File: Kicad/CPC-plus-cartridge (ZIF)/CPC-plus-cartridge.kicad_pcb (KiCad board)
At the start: 2 copper layers, 47.2 x 78.7 mm, 18 parts, among them J1 Amstrad-CPC-plus-cartridge, J2 JTAG, U1 SST39SF040, U2 XC9536XL-VQ44, U3 SPX3819M5-L-3-3, U4 XC6206PxxxMR

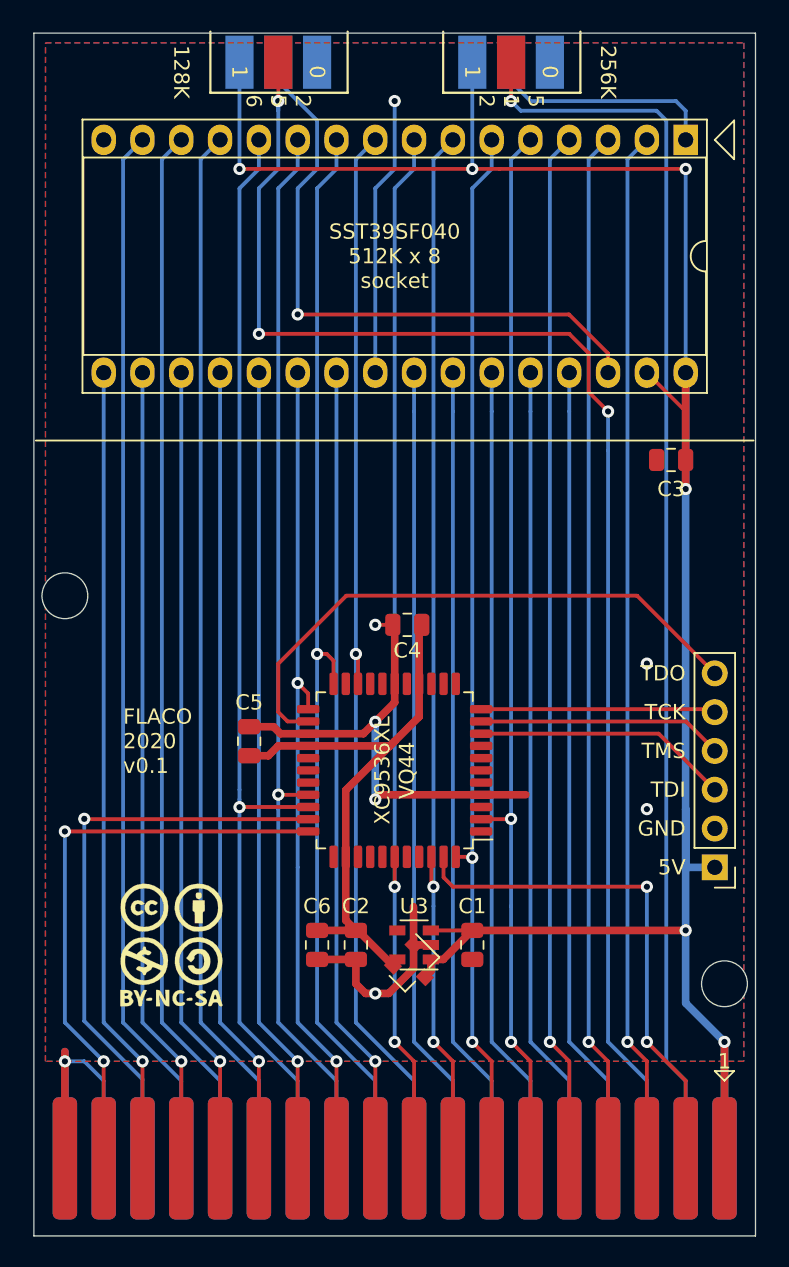
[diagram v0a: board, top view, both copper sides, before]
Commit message: Photo, InteractiveHtmlBom and README
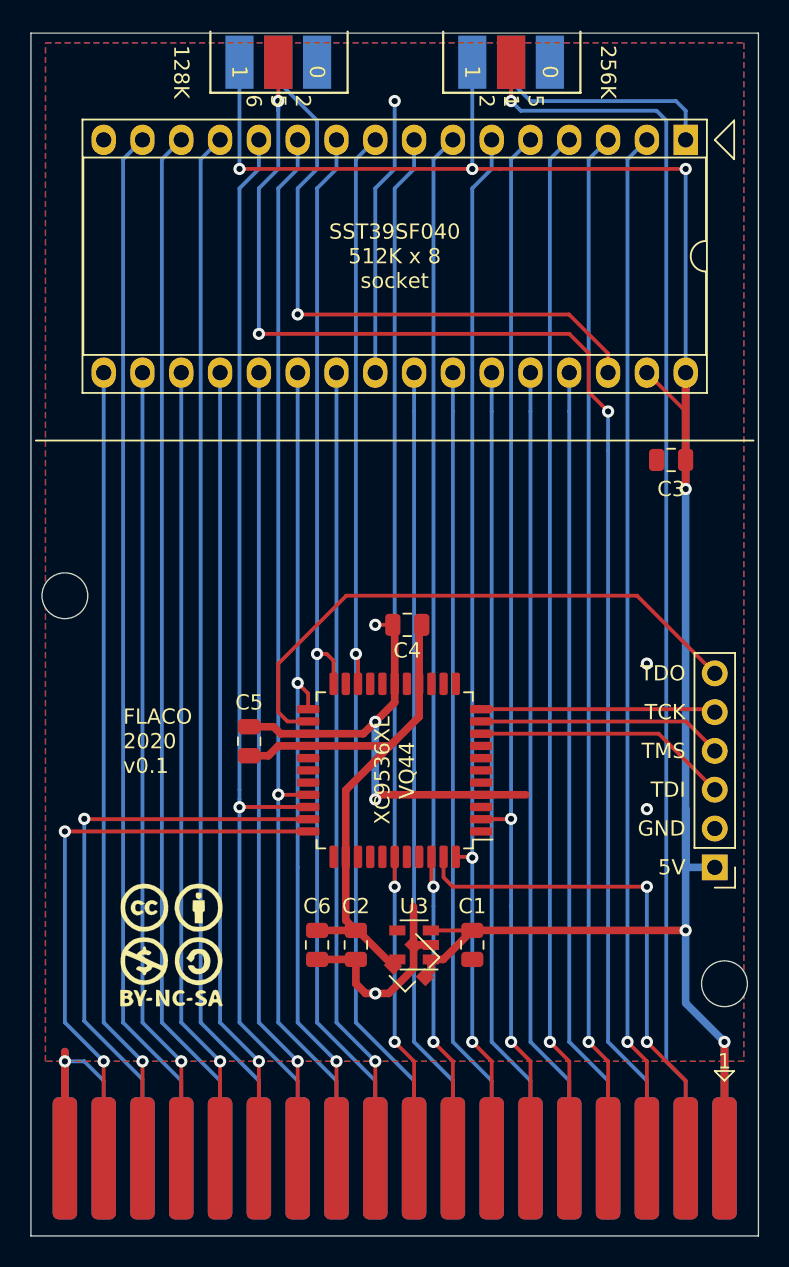
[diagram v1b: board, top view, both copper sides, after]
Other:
- board size 47.2 x 78.7 mm -> 47.6 x 78.7 mm
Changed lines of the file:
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@@
-(kicad_pcb (version 20171130) (host pcbnew 5.1.8-db9833491~88~ubuntu20.04.1)
+(kicad_pcb (version 20171130) (host pcbnew 5.1.12-84ad8e8a86~92~ubuntu20.04.1)
   (general
     (thickness 1.6)
@@
   )
   (page A4)
+  (title_block
+    (title "CPC plus cartridge (ZIF)")
+    (date 2021-12-11)
+    (rev 0.2)
+    (company "FLACO 2019-2020, licence of this schematic is CC-BY-NC-SA")
+    (comment 1 "from 0.1: slight width increase to better fit the CPC connector")
+  )
   (layers
     (0 F.Cu signal)
@@
       (effects (font (size 1 1) (thickness 0.15)))
     )
+    (fp_circle (center 0 0) (end 3 0) (layer Cmts.User) (width 0.15))
+    (fp_circle (center 0 0) (end 3.25 0) (layer F.CrtYd) (width 0.05))
     (fp_text user %R (at 0.3 0) (layer F.Fab)
       (effects (font (size 1 1) (thickness 0.15)))
     )
-    (fp_circle (center 0 0) (end 3 0) (layer Cmts.User) (width 0.15))
-    (fp_circle (center 0 0) (end 3.25 0) (layer F.CrtYd) (width 0.05))
     (pad 1 np_thru_hole circle (at 0 0) (size 3 3) (drill 3) (layers *.Cu *.Mask))
   )
@@
       (effects (font (size 1 1) (thickness 0.15)))
     )
+    (fp_circle (center 0 0) (end 3 0) (layer Cmts.User) (width 0.15))
+    (fp_circle (center 0 0) (end 3.25 0) (layer F.CrtYd) (width 0.05))
     (fp_text user %R (at 0.3 0) (layer F.Fab)
       (effects (font (size 1 1) (thickness 0.15)))
     )
-    (fp_circle (center 0 0) (end 3 0) (layer Cmts.User) (width 0.15))
-    (fp_circle (center 0 0) (end 3.25 0) (layer F.CrtYd) (width 0.05))
     (pad 1 np_thru_hole circle (at 0 0) (size 3 3) (drill 3) (layers *.Cu *.Mask))
   )
@@
       (effects (font (size 1 1) (thickness 0.15)))
     )
-    (fp_text user "PCB Edge" (at -7.54 1) (layer Dwgs.User)
-      (effects (font (size 0.5 0.5) (thickness 0.125)))
-    )
     (fp_line (start -8.54 2) (end 8.255 2) (layer Dwgs.User) (width 0.15))
     (fp_line (start -4.54 2) (end -4.54 -2) (layer F.SilkS) (width 0.15))
     (fp_line (start -4.54 -2) (end 4.445 -2) (layer F.SilkS) (width 0.15))
     (fp_line (start 4.445 -2) (end 4.445 2) (layer F.SilkS) (width 0.15))
+    (fp_text user "PCB Edge" (at -7.54 1) (layer Dwgs.User)
+      (effects (font (size 0.5 0.5) (thickness 0.125)))
+    )
     (pad 4 smd rect (at 0 0 180) (size 1.846667 3.48) (layers F.Cu F.Paste F.Mask)
       (net 31 /A18))
@@
       (effects (font (size 1 1) (thickness 0.15)))
     )
-    (fp_text user "PCB Edge" (at -7.54 1) (layer Dwgs.User)
-      (effects (font (size 0.5 0.5) (thickness 0.125)))
-    )
     (fp_line (start -8.54 2) (end 8.255 2) (layer Dwgs.User) (width 0.15))
     (fp_line (start -4.54 2) (end -4.54 -2) (layer F.SilkS) (width 0.15))
     (fp_line (start -4.54 -2) (end 4.445 -2) (layer F.SilkS) (width 0.15))
     (fp_line (start 4.445 -2) (end 4.445 2) (layer F.SilkS) (width 0.15))
+    (fp_text user "PCB Edge" (at -7.54 1) (layer Dwgs.User)
+      (effects (font (size 0.5 0.5) (thickness 0.125)))
+    )
     (pad 4 smd rect (at 0 0 180) (size 1.846667 3.48) (layers F.Cu F.Paste F.Mask)
       (net 29 /A17))
@@
     (arrow2b (pts (xy 122.555 82.55) (xy 121.968579 81.423496)))
   )
-  (gr_line (start 130.048 55.88) (end 177.292 55.88) (layer Edge.Cuts) (width 0.05))
-  (gr_line (start 130.048 134.62) (end 130.048 55.88) (layer Edge.Cuts) (width 0.05))
-  (gr_line (start 177.292 134.62) (end 177.292 55.88) (layer Edge.Cuts) (width 0.05))
+  (gr_line (start 129.8575 55.88) (end 177.4825 55.88) (layer Edge.Cuts) (width 0.05))
+  (gr_line (start 129.8575 134.62) (end 129.8575 55.88) (layer Edge.Cuts) (width 0.05))
+  (gr_line (start 177.4825 134.62) (end 177.4825 55.88) (layer Edge.Cuts) (width 0.05))
   (dimension 47.244 (width 0.15) (layer Dwgs.User)
     (gr_text "47,244 mm" (at 153.67 147.348048) (layer Dwgs.User)
@@
   (gr_line (start 177.292 125.476) (end 179.832 125.476) (layer Dwgs.User) (width 0.05))
   (gr_line (start 177.292 134.62) (end 177.292 125.476) (layer Dwgs.User) (width 0.05))
-  (gr_line (start 130.048 134.62) (end 177.292 134.62) (layer Edge.Cuts) (width 0.05))
+  (gr_line (start 129.8575 134.62) (end 177.4825 134.62) (layer Edge.Cuts) (width 0.05))
   (gr_line (start 130.048 125.476) (end 130.048 134.62) (layer Dwgs.User) (width 0.05))
   (gr_line (start 127.508 125.476) (end 130.048 125.476) (layer Dwgs.User) (width 0.05))
